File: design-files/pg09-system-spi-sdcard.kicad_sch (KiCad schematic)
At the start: 1 part, among them U1001 W65C22

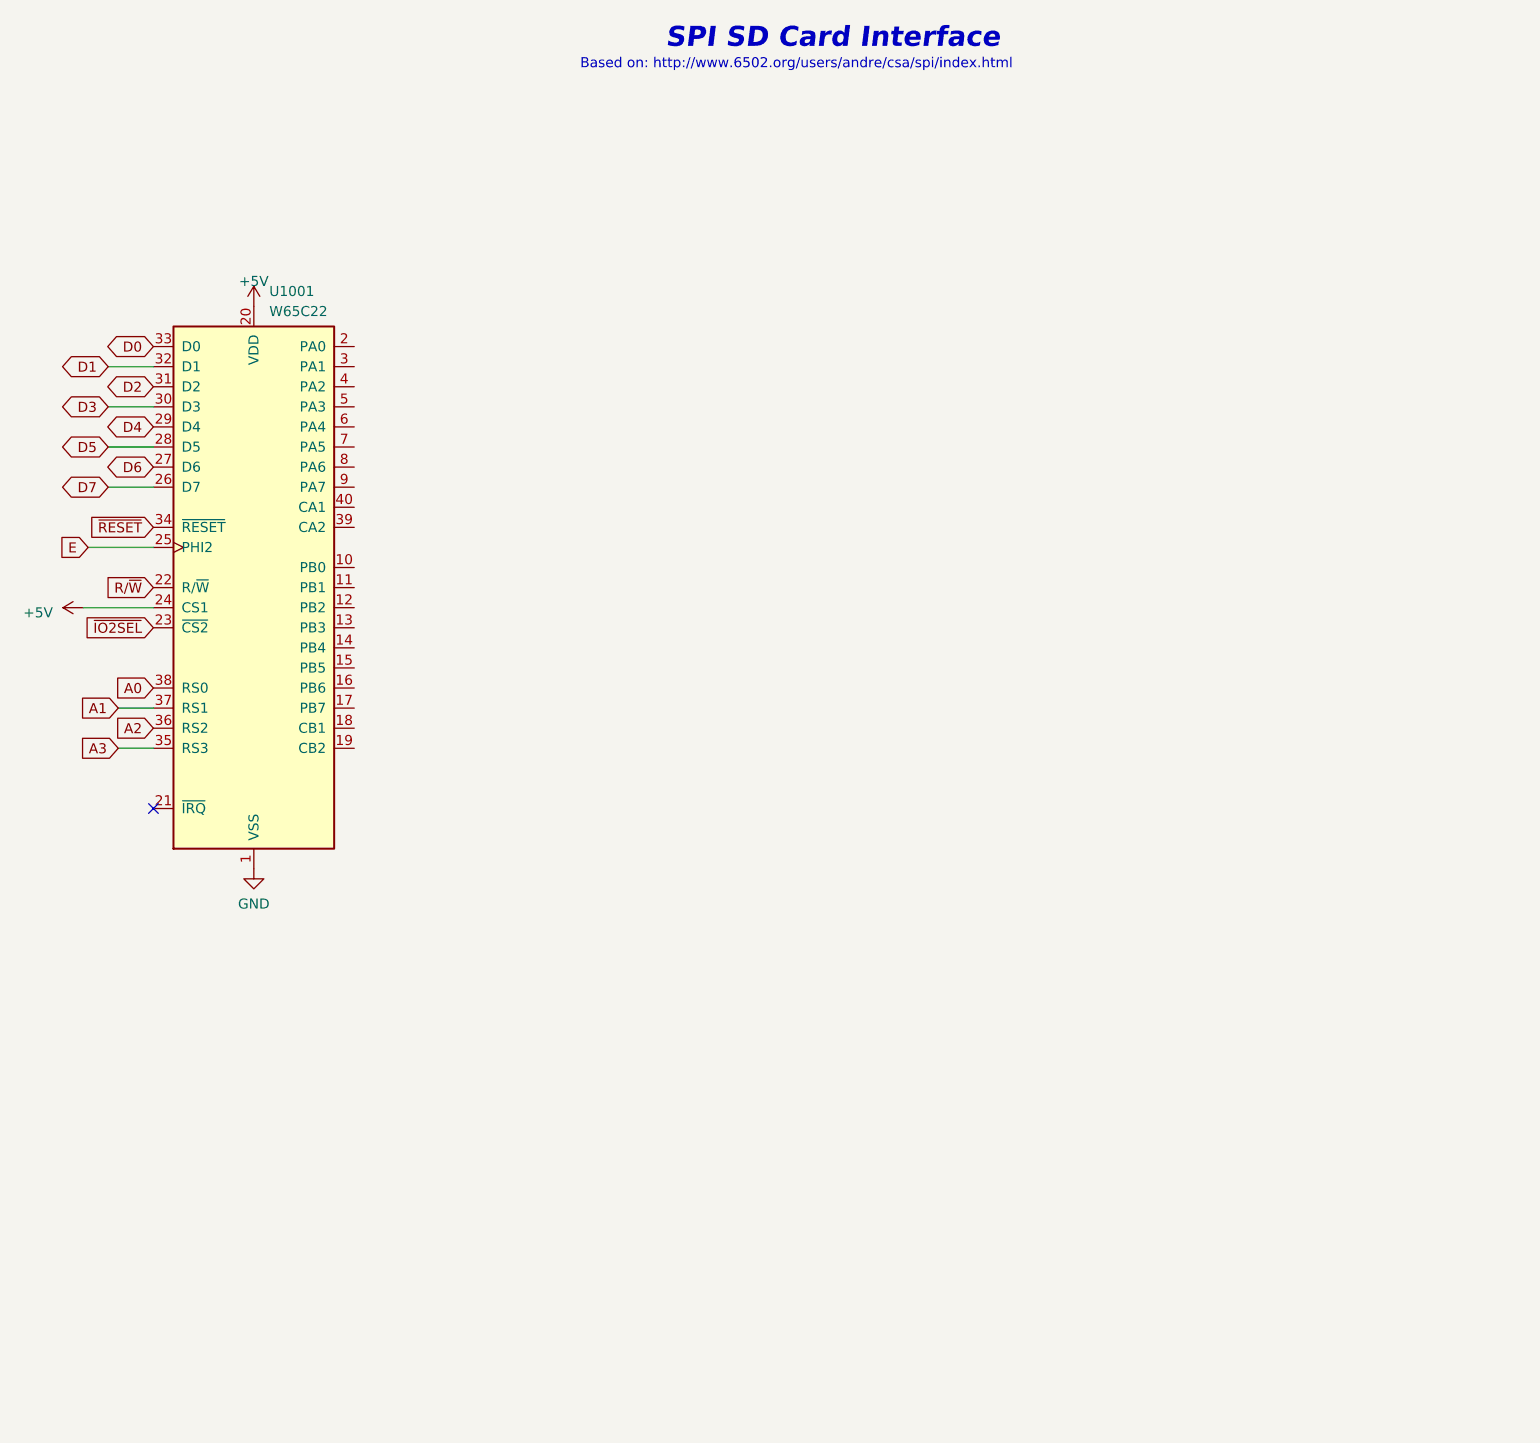
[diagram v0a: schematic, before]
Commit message: Move Reset to the main sheet.  Checkpoint SD Card SPI interface.
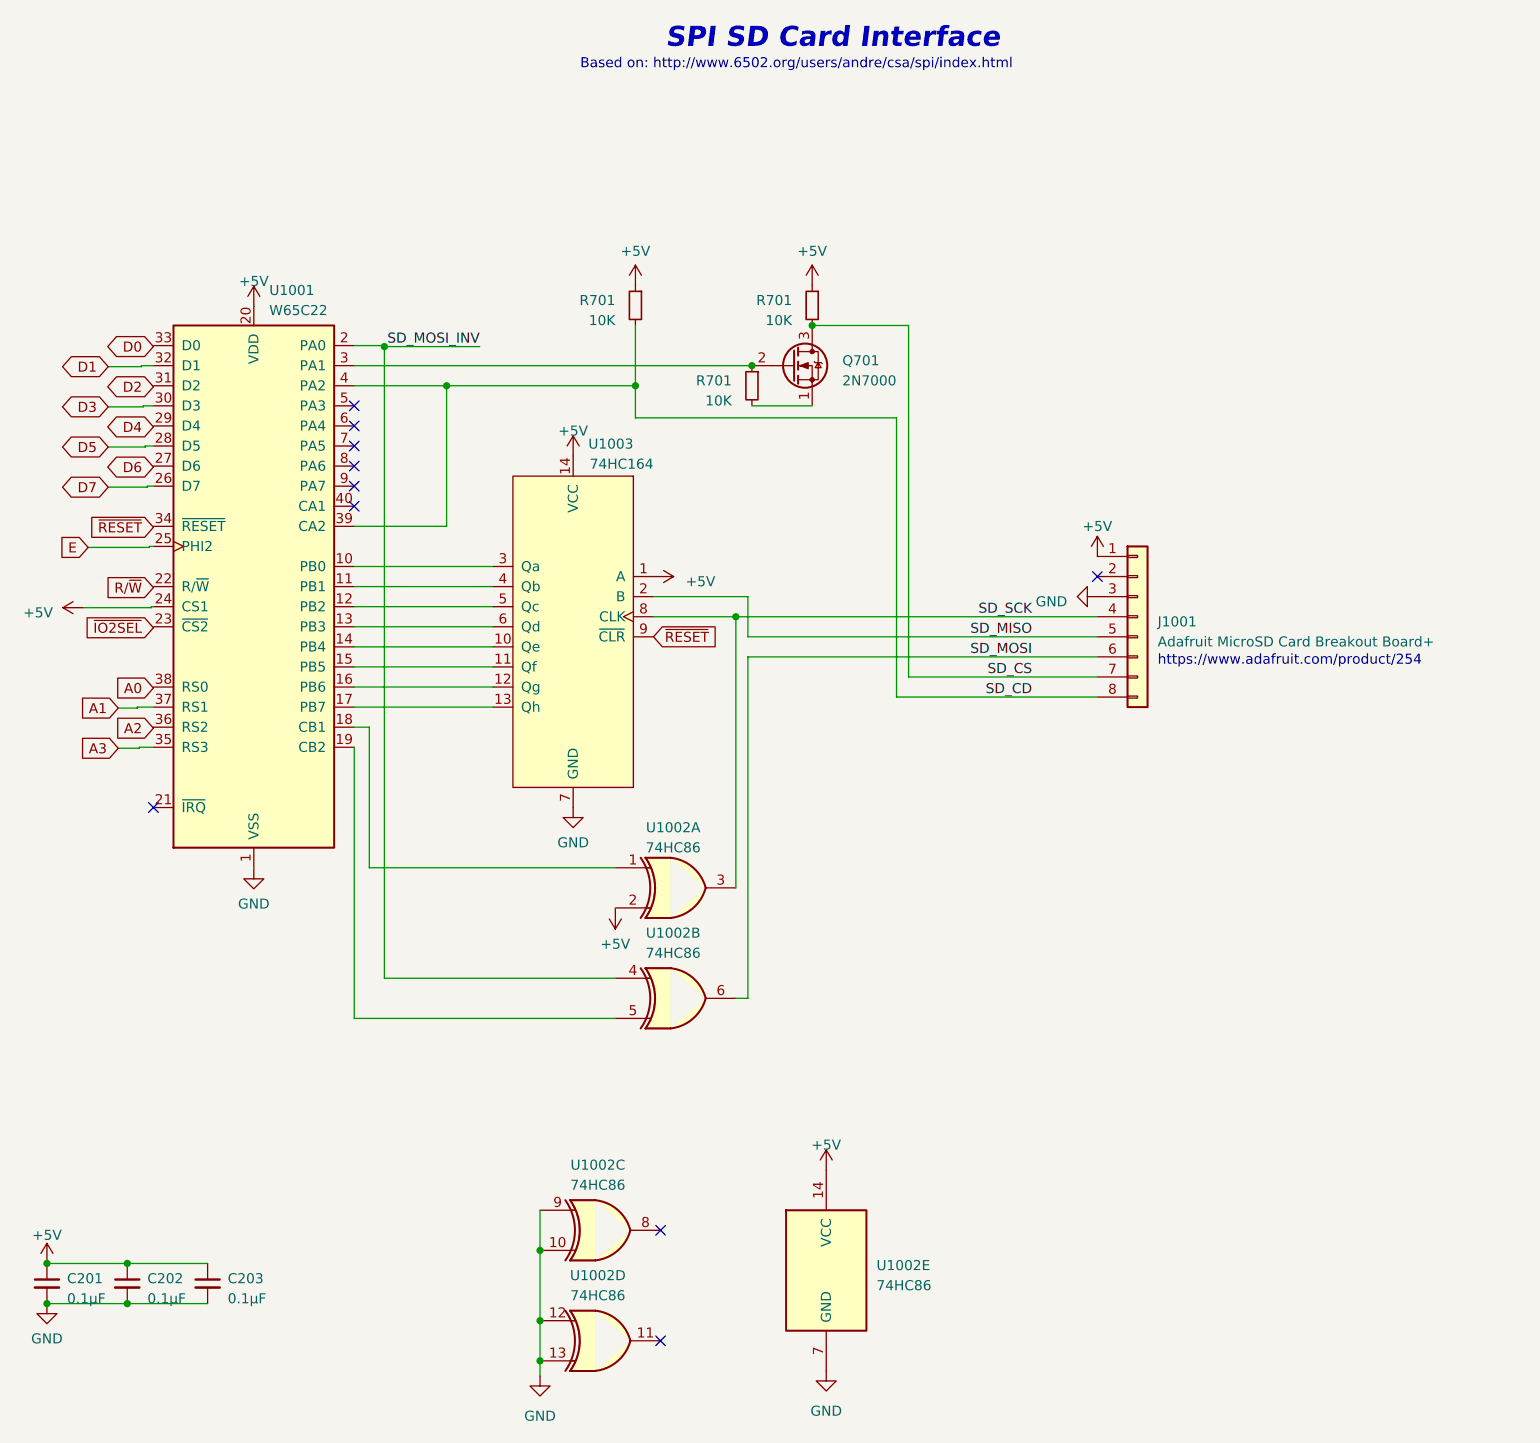
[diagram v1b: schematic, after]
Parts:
- added C201, C202, C203: 0.1µF, Capacitor_THT:C_Disc_D3.8mm_W2.6mm_P2.50mm, symbol Device:C_Small
- added J1001: Adafruit MicroSD Card Breakout Board+, Connector_PinHeader_2.54mm:PinHeader_1x08_P2.54mm_Vertical, symbol Connector_Generic:Conn_01x08
- added Q701: 2N7000, Package_TO_SOT_THT:TO-92_Inline, symbol Transistor_FET:2N7000
- added R701 (x3): 10K, Resistor_THT:R_Axial_DIN0207_L6.3mm_D2.5mm_P7.62mm_Horizontal, symbol Device:R_Small
- added U1002: 74HC86, Package_DIP:DIP-14_W7.62mm_Socket, symbol 74xx:74HC86
- added U1003: 74HC164, Package_DIP:DIP-14_W7.62mm_Socket, symbol jrt-ICs:74LS164
- U1001: footprint Package_DIP:DIP-40_W15.24mm -> Package_DIP:DIP-40_W15.24mm_Socket
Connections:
- net +5V: now also C201.1, C202.1, C203.1, J1001.1 (Pin_1), R701.1, R701.1, U1002.14 (VCC), U1002.2, U1003.1 (A), U1003.14 (VCC)
- net GND: now also C201.2, C202.2, C203.2, J1001.3 (Pin_3), U1002.10, U1002.12, U1002.13, U1002.7 (GND), U1002.9, U1003.7 (GND)
- net ~{RESET}: now also U1003.9 (~{CLR})
- net at U1001.10 (PB0): now also U1003.3 (Qa)
- net at U1001.11 (PB1): now also U1003.4 (Qb)
- net at U1001.12 (PB2): now also U1003.5 (Qc)
- net at U1001.13 (PB3): now also U1003.6 (Qd)
- net at U1001.14 (PB4): now also U1003.10 (Qe)
- net at U1001.15 (PB5): now also U1003.11 (Qf)
- net at U1001.16 (PB6): now also U1003.12 (Qg)
- net at U1001.17 (PB7): now also U1003.13 (Qh)
- net at U1001.18 (CB1): now also U1002.1
- net at U1001.19 (CB2): now also U1002.5
- net SD_MOSI_INV: now reaches U1001.2 (PA0)
- net SD_MOSI_INV: now also U1002.4
- net at U1001.3 (PA1): now also Q701.2 (G), R701.1
- net SD_CD: now reaches U1001.39 (CA2)
- net SD_CD: now also U1001.4 (PA2), J1001.8 (Pin_8), R701.2
- new net: Q701.1 (S), R701.2
- new net SD_CS: J1001.7 (Pin_7), Q701.3 (D), R701.2
- new net SD_MISO: J1001.5 (Pin_5), U1003.2 (B)
- new net SD_MOSI: J1001.6 (Pin_6), U1002.6
- new net SD_SCK: J1001.4 (Pin_4), U1002.3, U1003.8 (CLK)
- no-connect marks 1 -> 10
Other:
- note added: "https://www.adafruit.com/product/254"
